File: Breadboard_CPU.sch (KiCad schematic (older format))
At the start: 21 parts, among them Q101 2N2222, SW101 RST

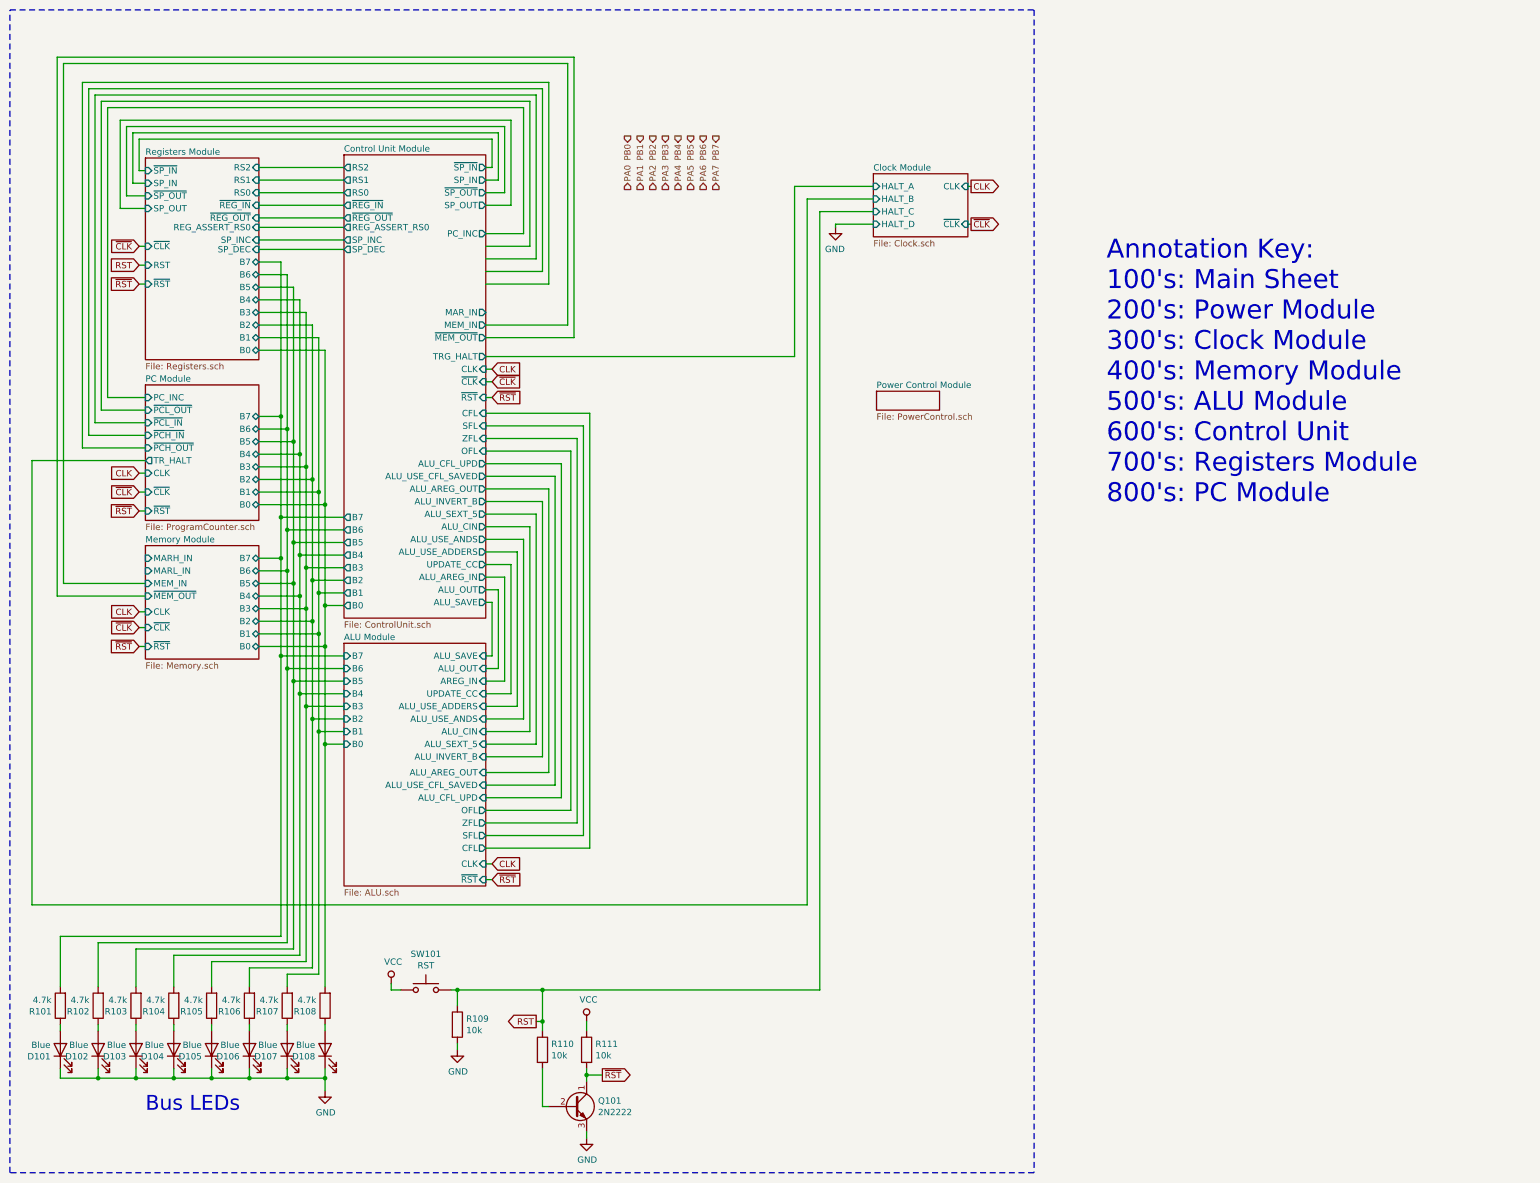
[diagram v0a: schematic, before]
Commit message: Testing memory module
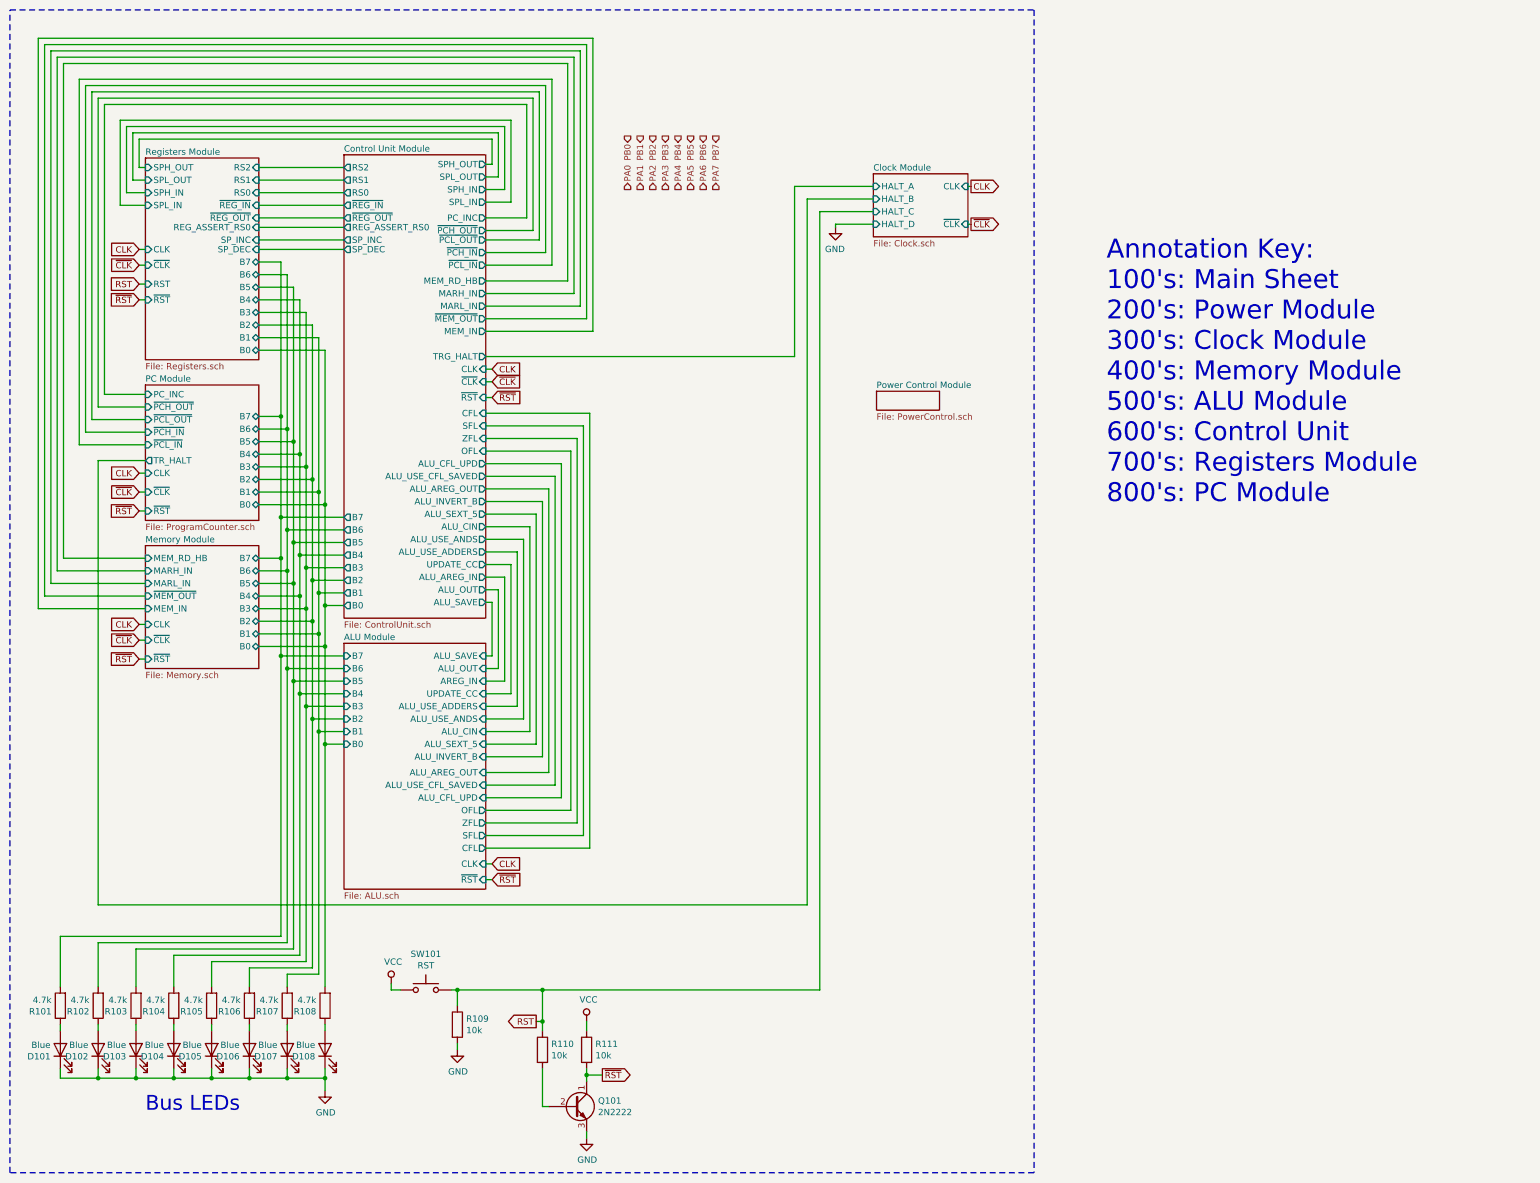
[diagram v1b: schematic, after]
